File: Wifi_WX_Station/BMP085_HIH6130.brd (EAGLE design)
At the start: 20.9 x 20.6 mm, 8 parts, among them U1 HIH_6130

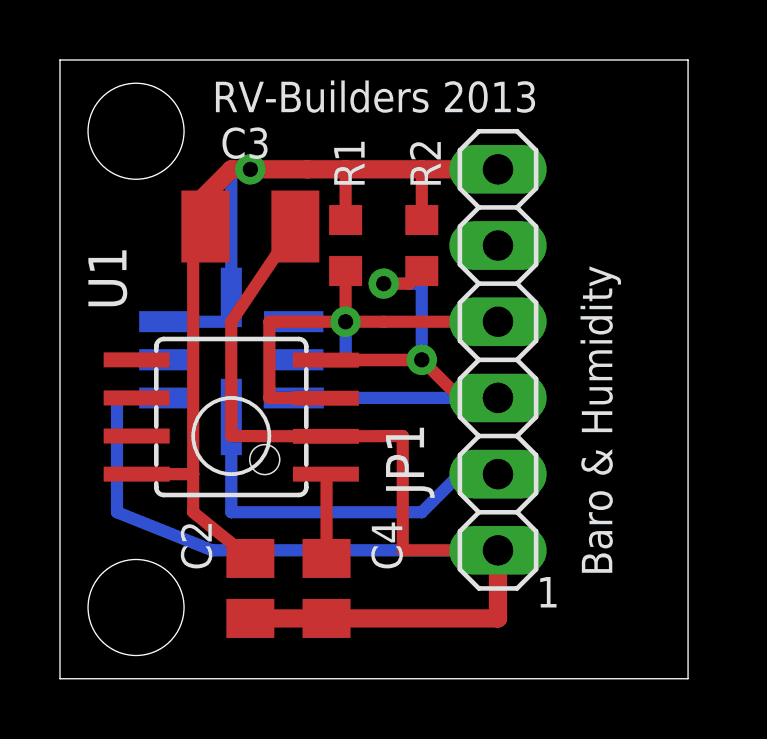
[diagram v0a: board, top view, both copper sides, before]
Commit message: updated BOM with all prices- As Checked in to BATCH PCB
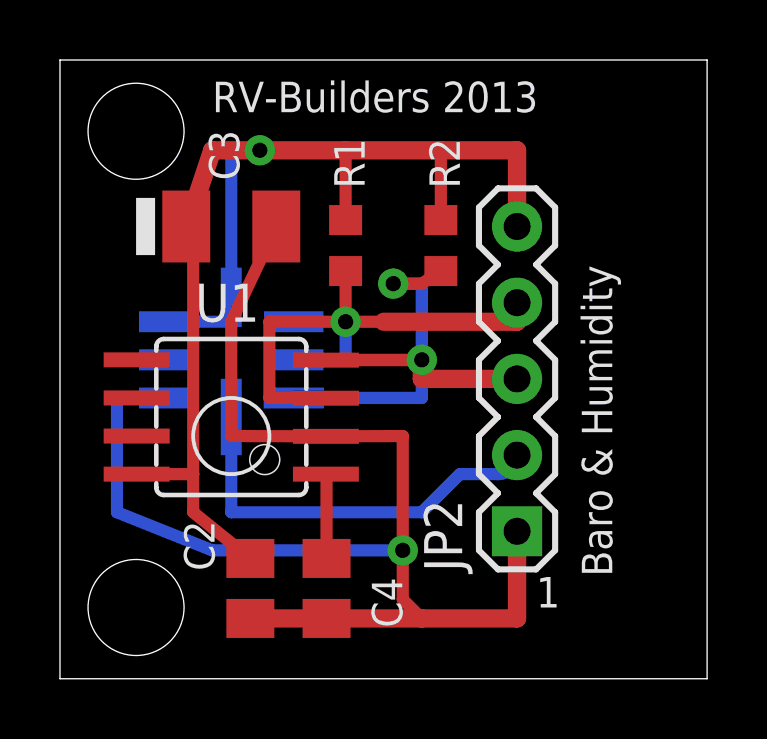
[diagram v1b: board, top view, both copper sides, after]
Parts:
- removed JP1: (no value), Headers:1X06
- added JP2: (no value), wifi_WX:1X05
- moved C3 0.63 mm to (11.4, 14.6)
- moved R2 0.63 mm to (18.4, 14.0)
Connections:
- net +3V3: now also JP2.5; no longer JP1.6
- net GND: now also JP2.1; no longer JP1.1
- net SCL: now also JP2.4; no longer JP1.4
- net SDA: now also JP2.3; no longer JP1.3
- net XCLR: now also JP2.2; no longer JP1.2
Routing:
- net +3V3: track 38.4 -> 43.3 mm
- net GND: track 49.3 -> 46.5 mm, vias 0 -> 1
- net SCL: track 16.7 -> 18.0 mm
- net XCLR: track 12.6 -> 13.5 mm
- net SDA: track 20.9 -> 20.3 mm
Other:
- board size 20.9 x 20.6 mm -> 21.6 x 20.6 mm
